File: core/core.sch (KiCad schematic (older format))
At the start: 0 parts

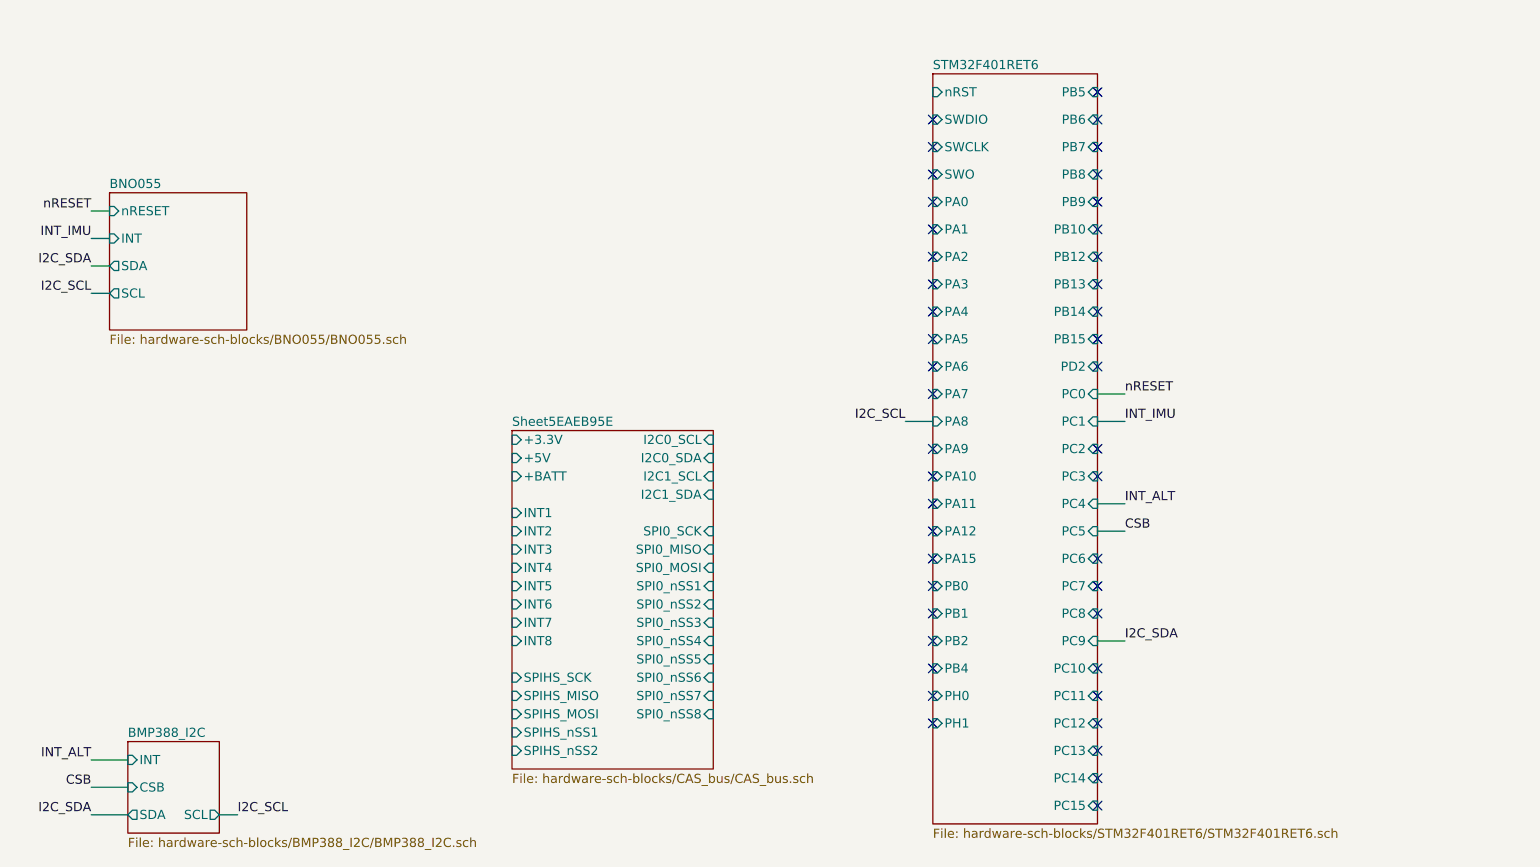
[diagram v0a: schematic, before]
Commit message: SPI/I2C boilerplate
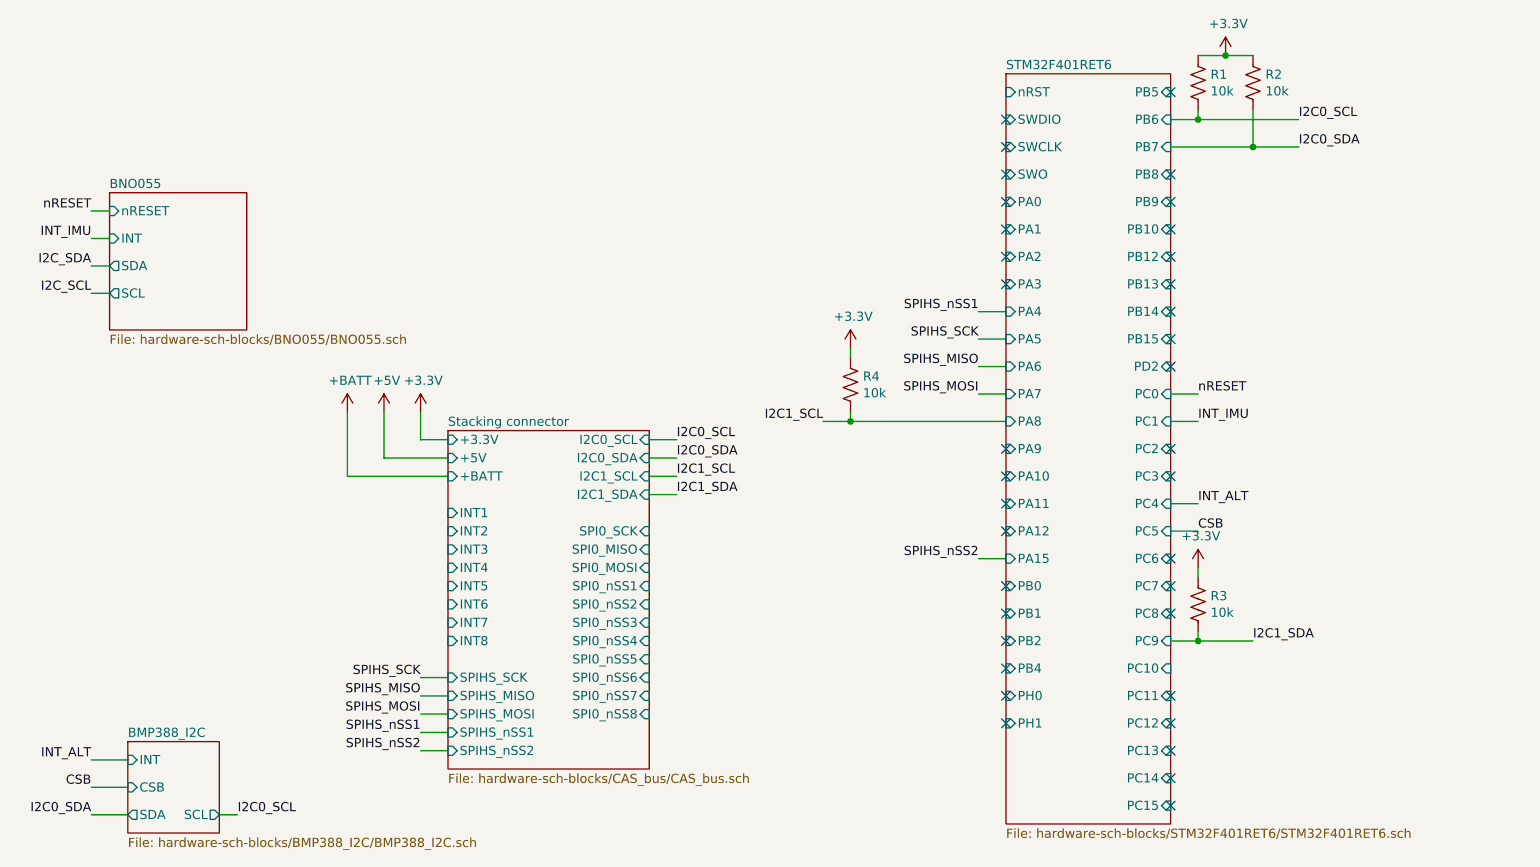
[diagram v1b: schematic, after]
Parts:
- added R1, R2, R3, R4: 10k, symbol Device:R_US
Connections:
- new net +3V3: R1.1, R2.1, R3.1, R4.1
- new net I2C0_SCL: R1.2
- new net I2C0_SDA: R2.2
- new net I2C1_SCL: R4.2
- new net I2C1_SDA: R3.2
- no-connect marks 44 -> 36
